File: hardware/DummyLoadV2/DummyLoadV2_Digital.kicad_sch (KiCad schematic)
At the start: 19 parts, among them J3 Display, J4 Digital, J7 Fan, Q3 2N7000, Q4 TP2104, SW1 Enable_SW, SW3 Range_SW, U1 Nano

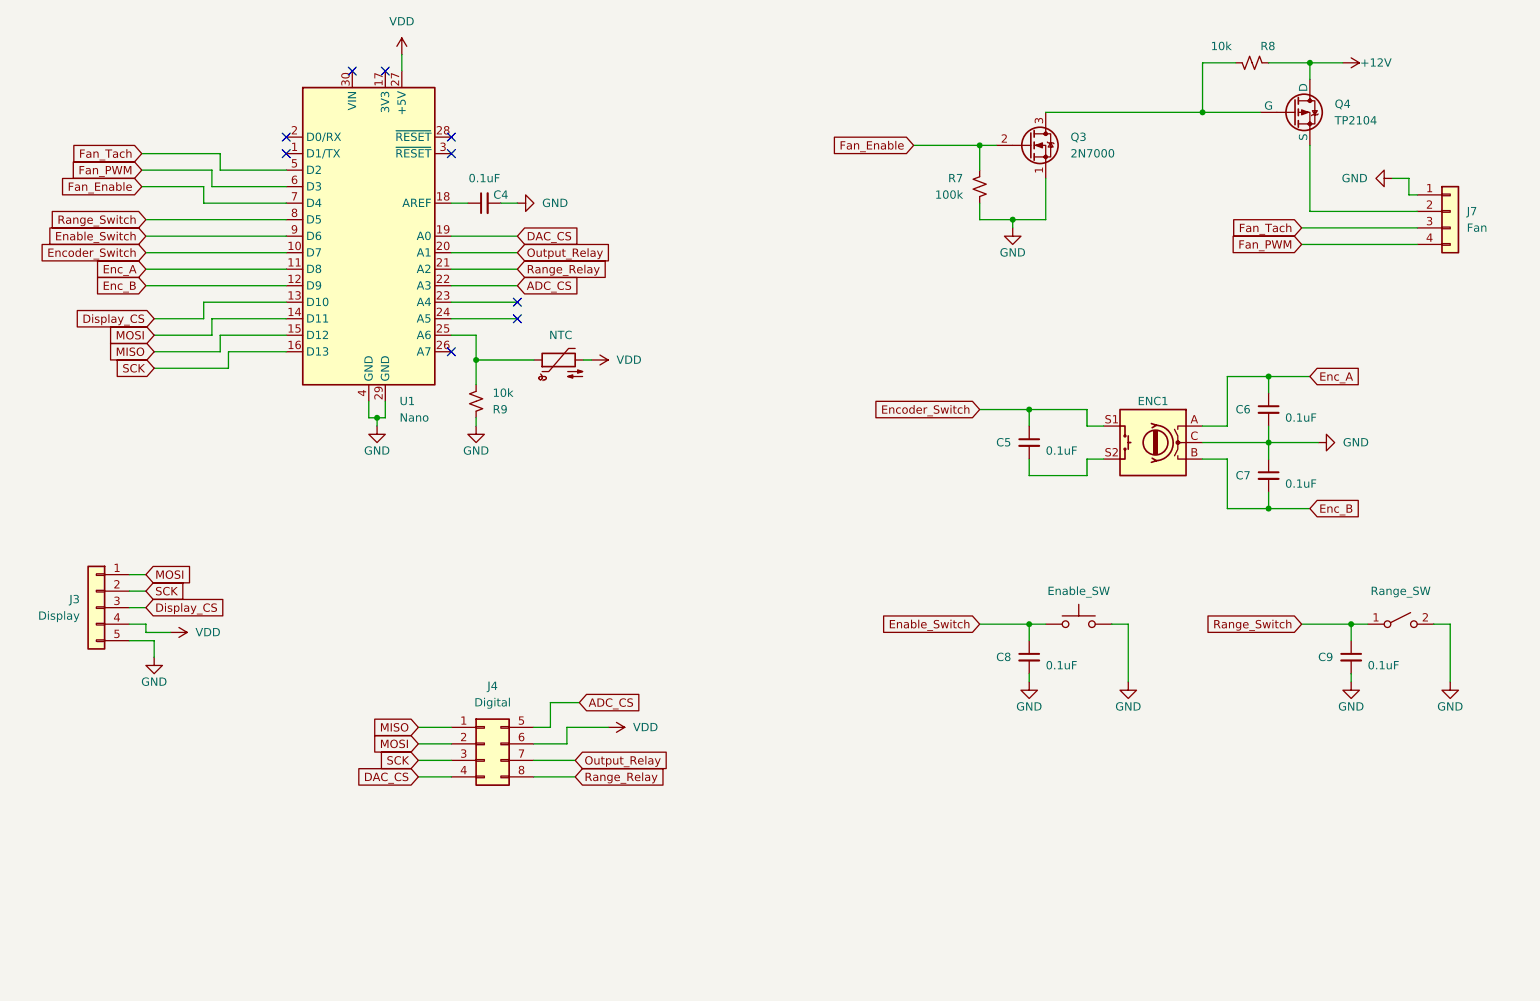
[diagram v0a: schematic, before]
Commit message: Updated schematic
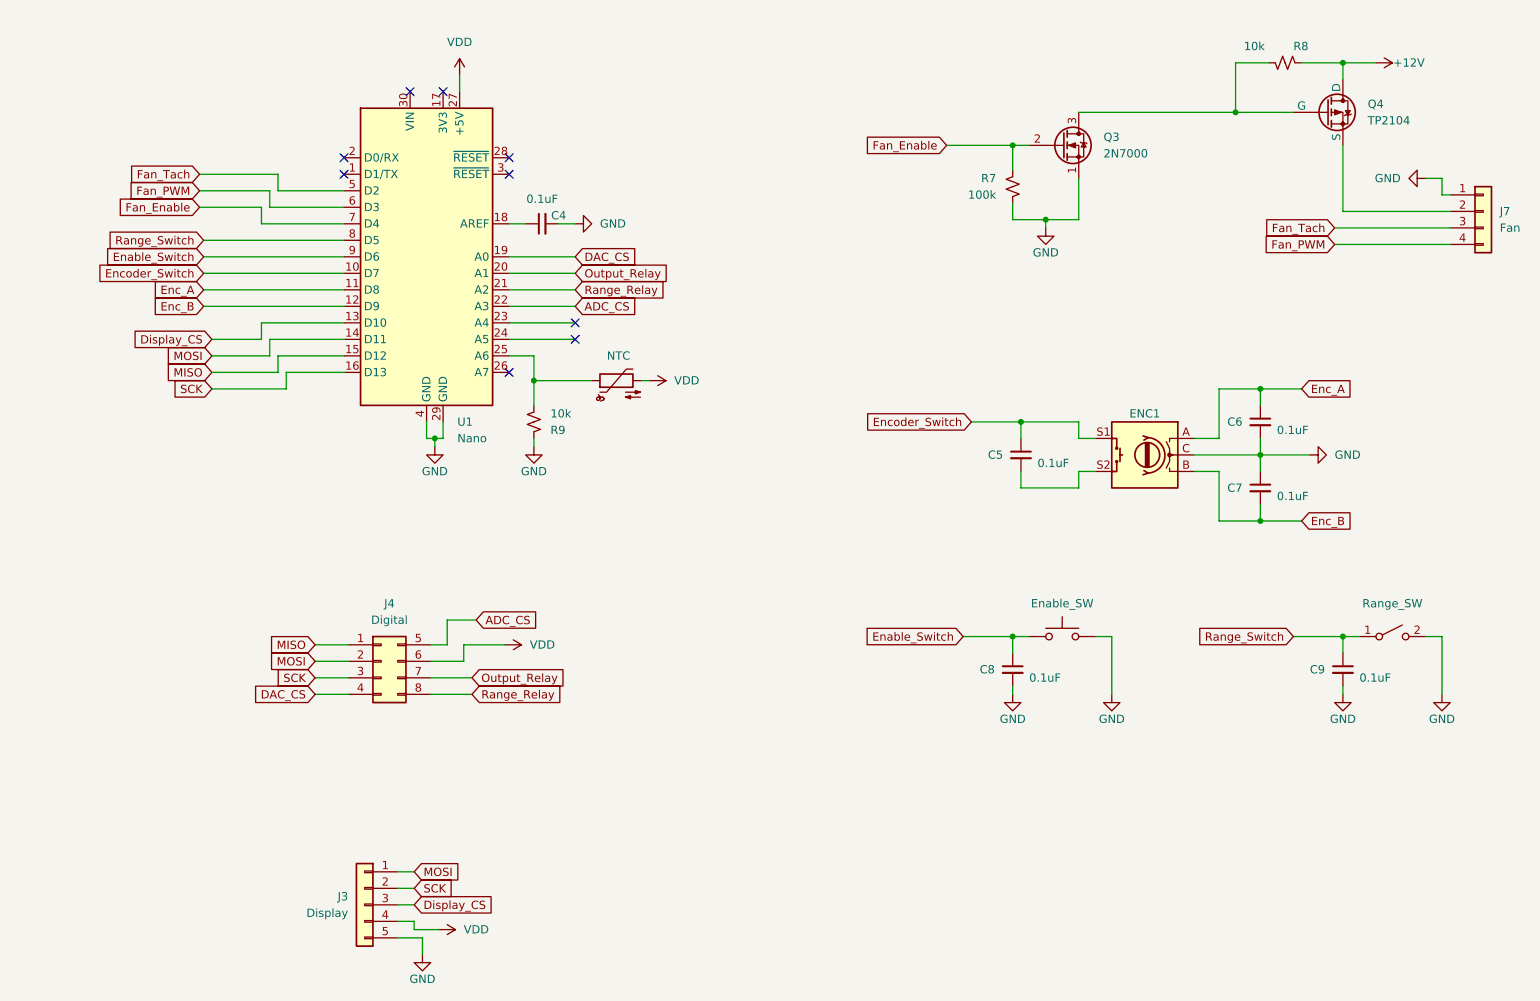
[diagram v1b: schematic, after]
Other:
- moved on the sheet: C4, C5, C6, C7, C8, C9, ENC1, J3, J4, J7, NTC, Q3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
